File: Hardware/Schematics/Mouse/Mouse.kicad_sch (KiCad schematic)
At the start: 17 parts, among them J1B Cable connector (fixed), J2 Controller Plug, SW1 Left, SW2 Right, U1 74HC04, U2 Vertical, U3 Horizontal, U4 74HC04

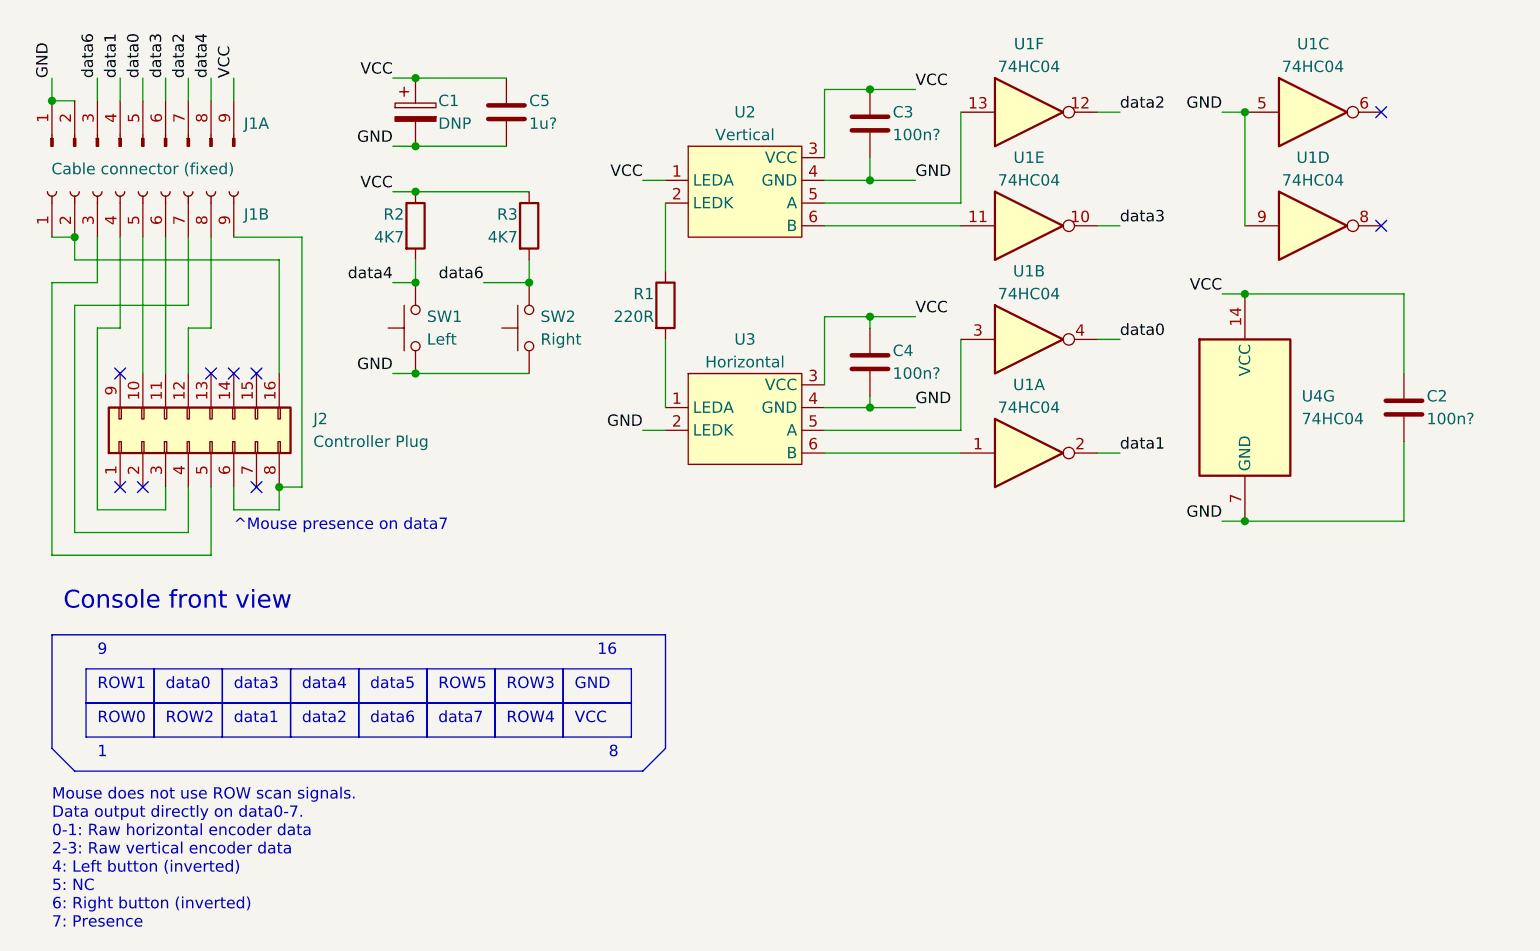
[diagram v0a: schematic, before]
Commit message: Mouse capacitors measured
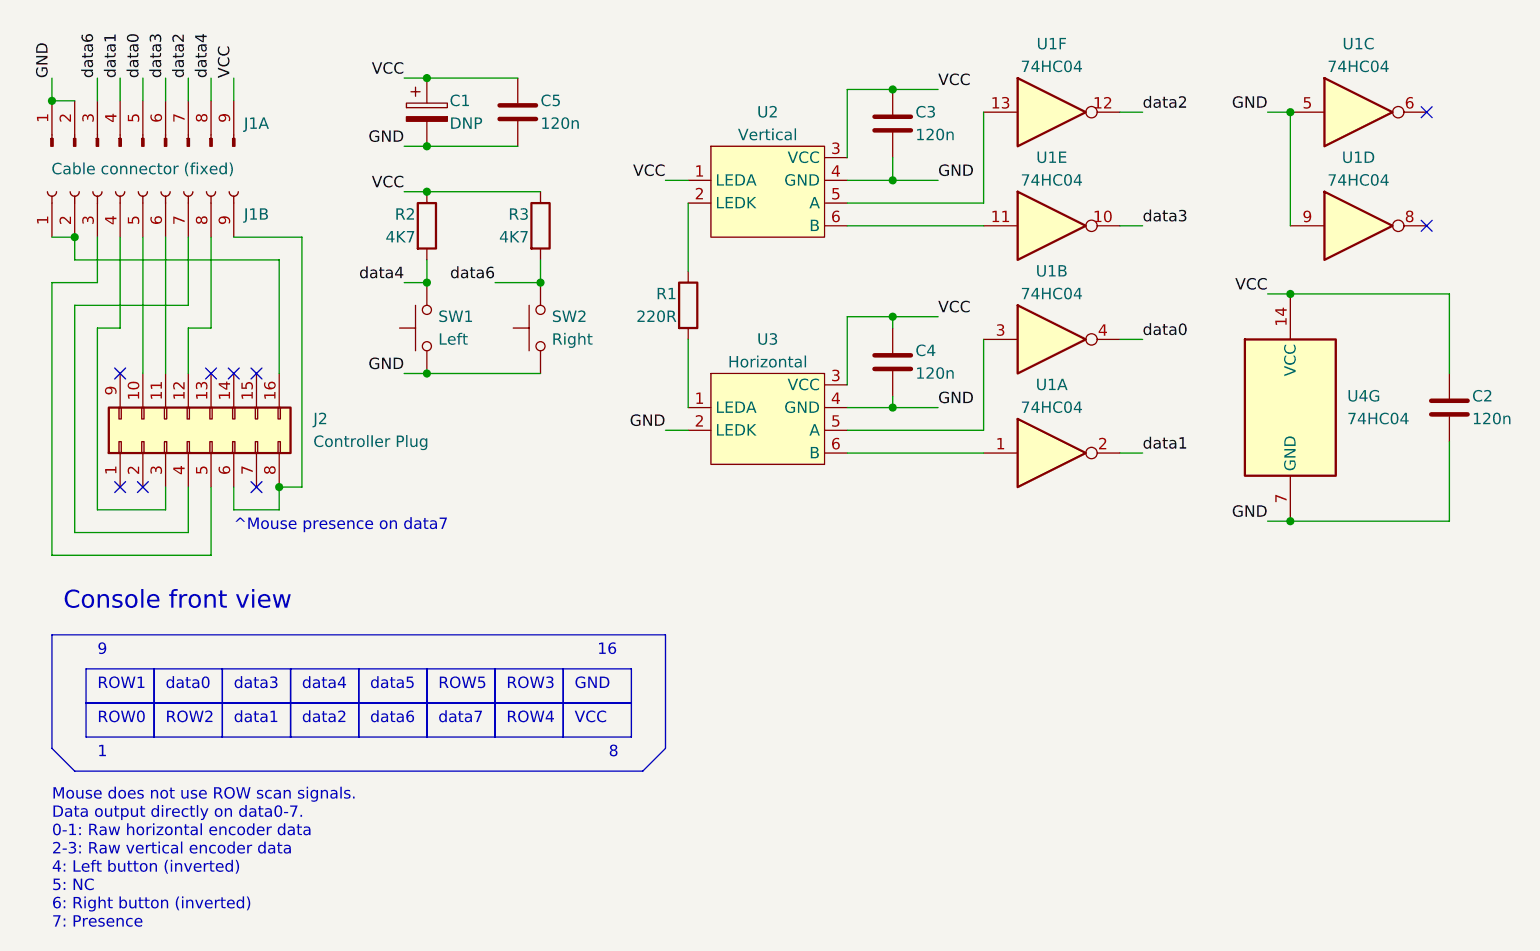
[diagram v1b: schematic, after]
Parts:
- C2, C3, C4: value 100n? -> 120n
- C5: value 1u? -> 120n
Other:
- moved on the sheet: C1, C2, C3, C4, C5, R1, R2, R3, SW1, SW2, U1A, U1B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
